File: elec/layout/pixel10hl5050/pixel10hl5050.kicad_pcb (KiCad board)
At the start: 2 copper layers, 2 parts

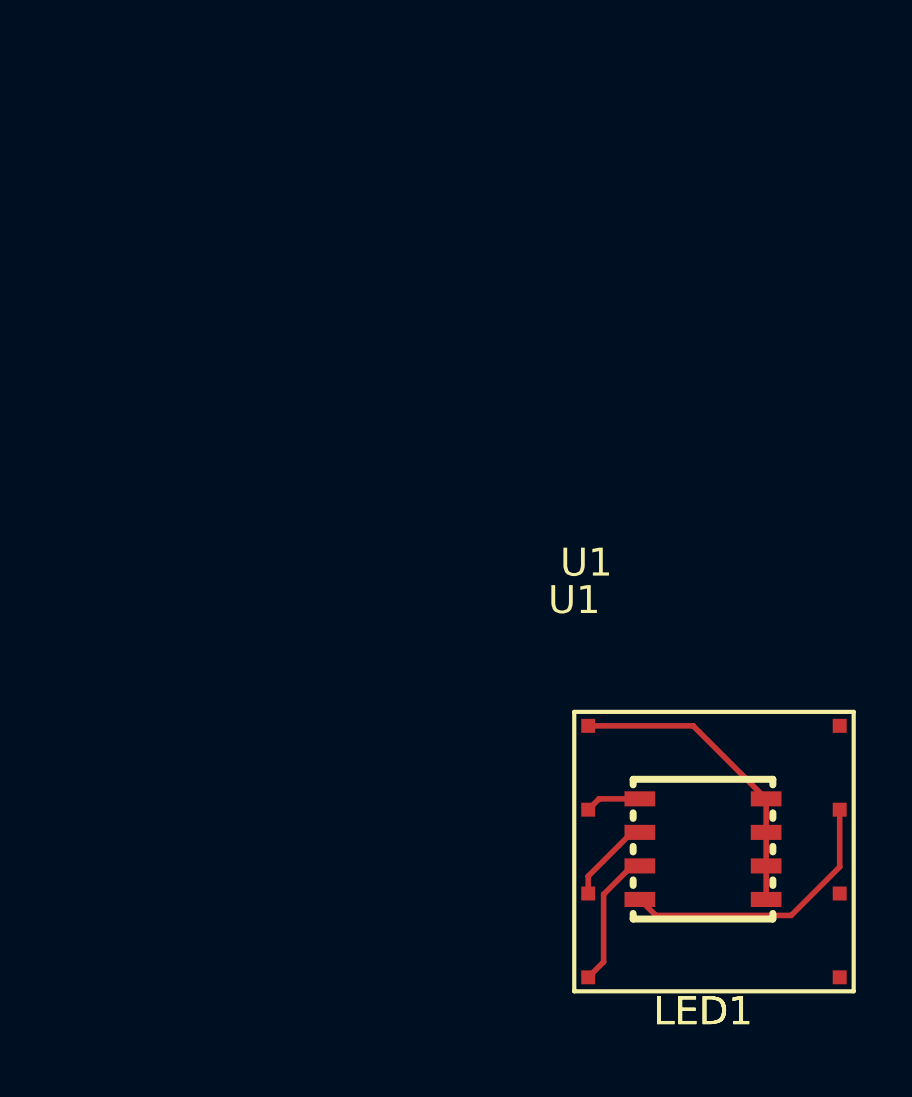
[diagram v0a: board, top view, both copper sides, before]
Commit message: pixel refactor
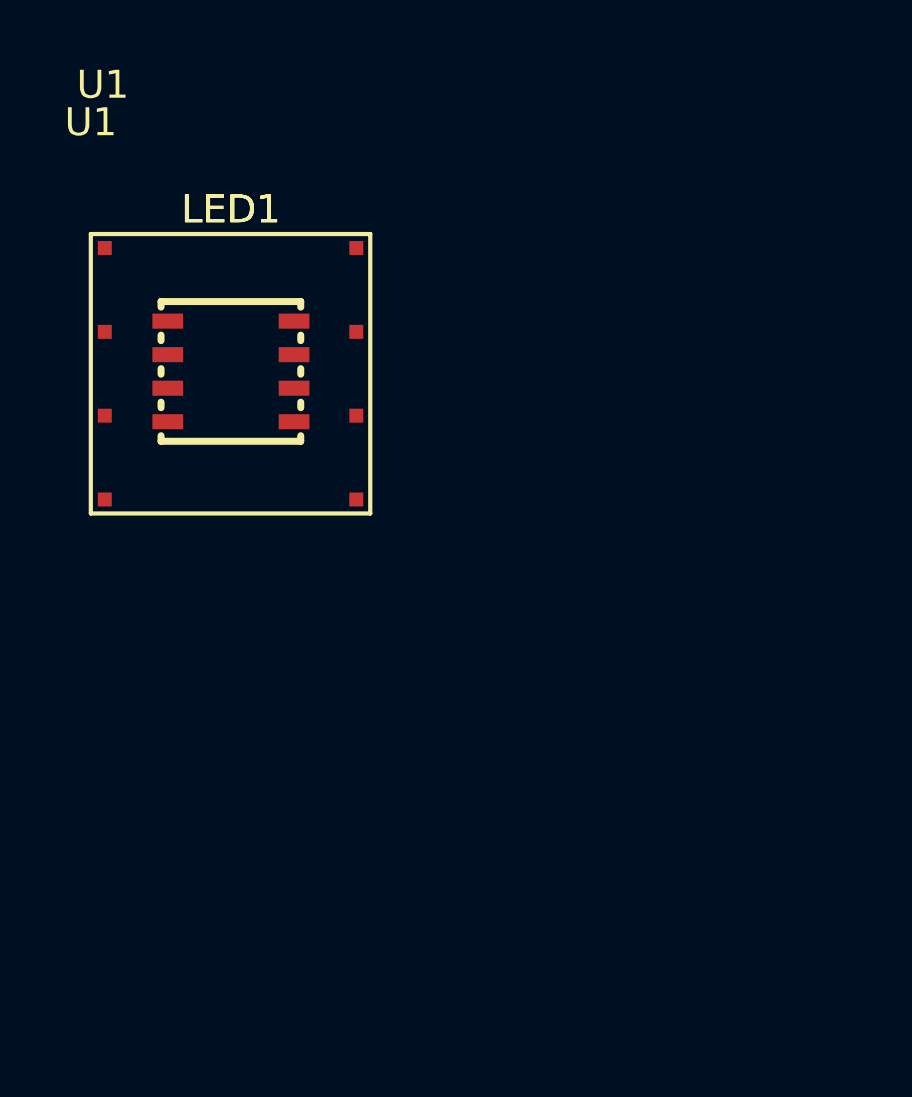
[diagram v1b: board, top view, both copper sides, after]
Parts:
- moved U1 24.3 mm to (0.00, 0.00)
- moved LED1 24.0 mm to (5.01, 4.92), turned to 0 degrees
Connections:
- net cathode_blue renamed blue
- net cathode_cold_white renamed cold_white
- net cathode_green renamed green
- net cathode_ir renamed ir
- net cathode_red renamed red
- net cathode_uv renamed uv
- net cathode_warm_white renamed warm_white
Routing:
- net anode: track 11.0 -> 0.00 mm
- net cold_white: track 10.2 -> 0.00 mm
- net blue: track 4.92 -> 0.00 mm
- net green: track 3.12 -> 0.00 mm
- net red: track 2.01 -> 0.00 mm

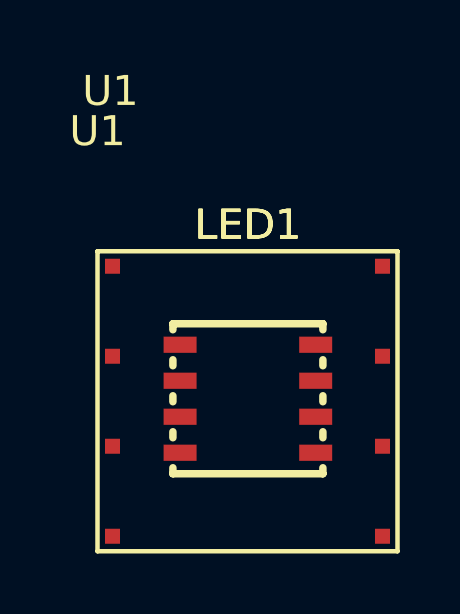
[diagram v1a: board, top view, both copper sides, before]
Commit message: updating rp2040
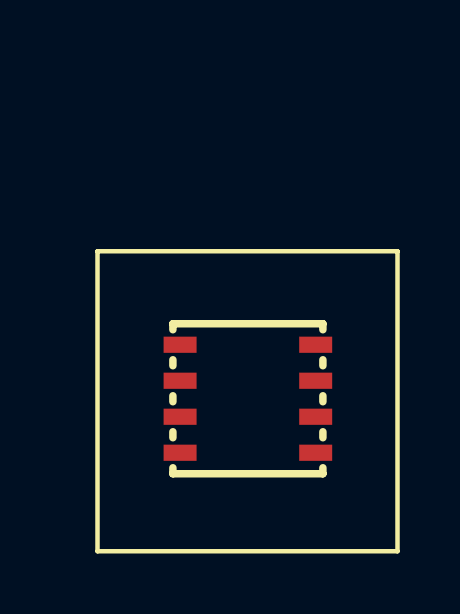
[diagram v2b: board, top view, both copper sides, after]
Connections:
- LED1 pad 1: cold_white -> rgb-cathodes-cathode-1
- LED1 pad 3: blue -> rgb-cathodes-cathode-0
- LED1 pad 5: green -> rgb-cathodes-cathode-2
- LED1 pad 7: red -> rgb-cathodes-cathode-3
